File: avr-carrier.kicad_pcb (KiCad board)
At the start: 2 copper layers, 1 part

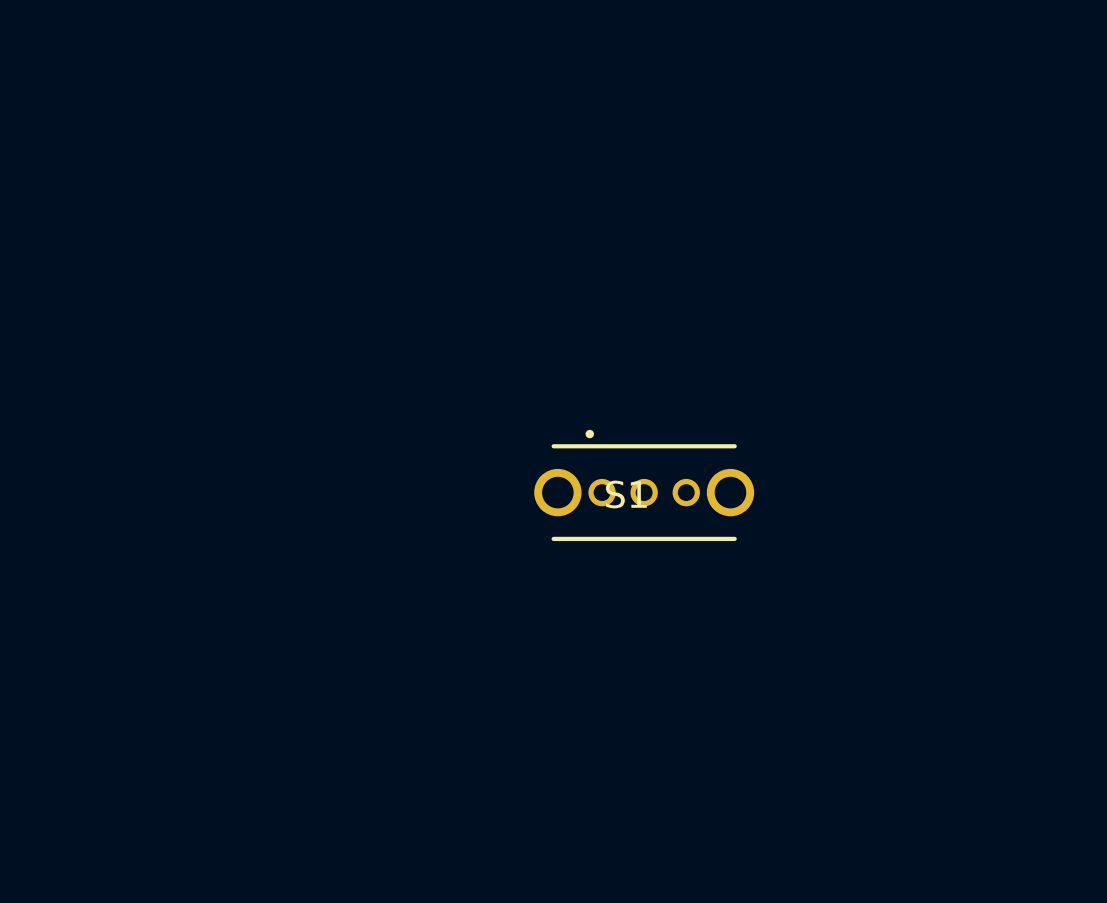
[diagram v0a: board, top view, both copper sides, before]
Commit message: hmm
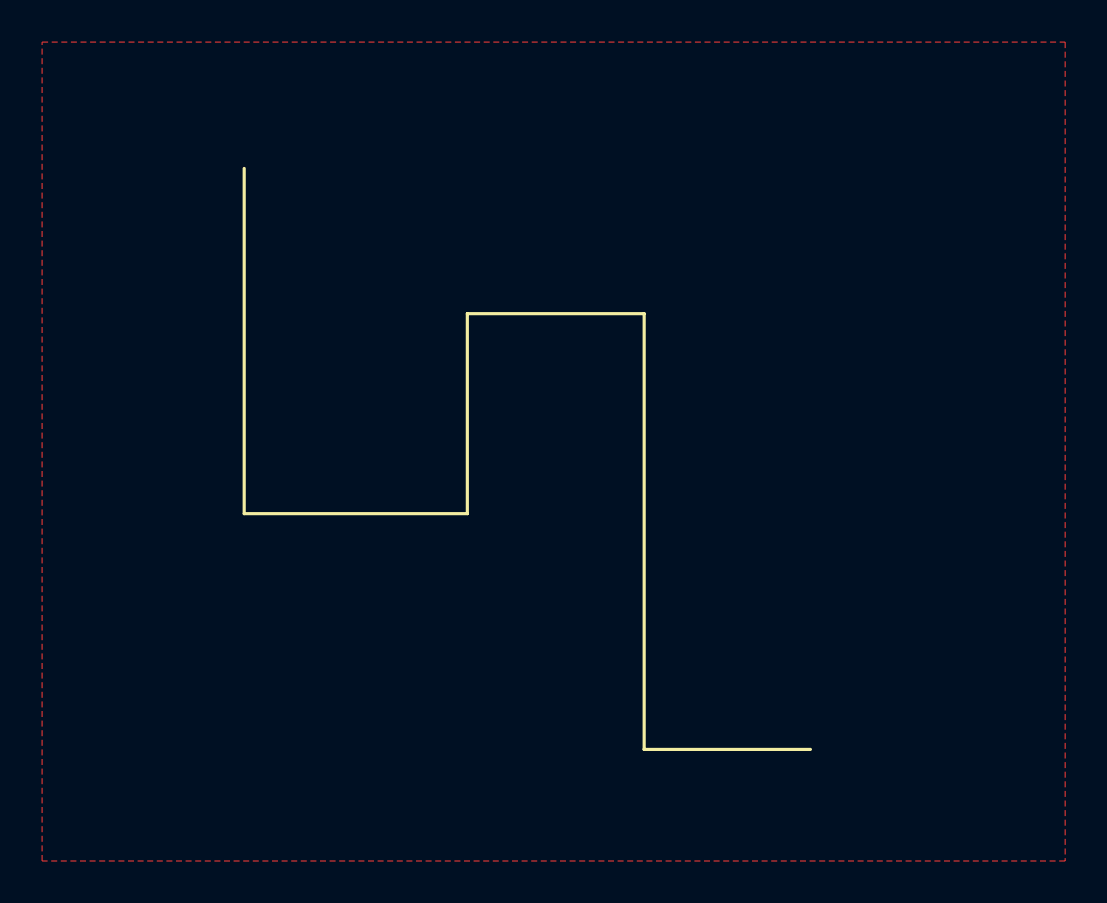
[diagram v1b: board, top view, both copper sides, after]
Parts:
- removed S1: OS102011MA1QN1, Switches_CC:OS102011MA1QN1
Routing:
- added copper zone on F.Cu, net (none)
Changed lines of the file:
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@@
   )
   (net 0 "")
-  (net 1 "unconnected-(S1-Pad1)")
-  (net 2 "unconnected-(S1-Pad2)")
-  (net 3 "unconnected-(S1-Pad3)")
-  (footprint "Switches_CC:OS102011MA1QN1" (layer "F.Cu")
-    (at 128.7 103.8)
-    (descr "OS102011MA1QN1")
-    (tags "Switch")
-    (property "Description" "Switch Slide Right Angle SPDT 0.1A 12VDC Through Hole Slide Switch SPDT On-On 0.1 A@ 12 V dc Slide")
-    (property "Height" "")
-    (property "Manufacturer_Name" "C & K COMPONENTS")
-    (property "Manufacturer_Part_Number" "OS102011MA1QN1")
-    (property "Mouser Part Number" "611-OS102011MA1QN1")
-    (property "Mouser Price/Stock" "https://www.mouser.co.uk/ProductDetail/CK/OS102011MA1QN1?qs=WtljUlYws5R6MUgHcLkz4w%3D%3D")
-    (property "Sheetfile" "avr-carrier.kicad_sch")
-    (property "Sheetname" "")
-    (attr through_hole)
-    (fp_text reference "S1" (at -0.822 0.137) (layer "F.SilkS")
-      (effects (font (size 1.27 1.27) (thickness 0.254)))
-    )
-    (fp_text value "OS102011MA1QN1" (at -0.822 0.137) (layer "F.SilkS") hide
-      (effects (font (size 1.27 1.27) (thickness 0.254)))
-    )
-    (fp_text user "${REFERENCE}" (at -0.822 0.137) (layer "F.Fab")
-      (effects (font (size 1.27 1.27) (thickness 0.254)))
-    )
-    (fp_line (start -4.3 -2.2) (end 4.3 -2.2) (layer "F.SilkS") (width 0.2))
-    (fp_line (start -4.3 2.2) (end 4.3 2.2) (layer "F.SilkS") (width 0.2))
-    (fp_circle (center -2.583 -2.781) (end -2.583 -2.68172) (layer "F.SilkS") (width 0.2) (fill none))
-    (fp_line (start -4.3 2.2) (end -4.3 -2.2) (layer "F.Fab") (width 0.2))
-    (fp_line (start -4.3 -2.2) (end 4.3 -2.2) (layer "F.Fab") (width 0.2))
-    (fp_line (start 4.3 -2.2) (end 4.3 2.2) (layer "F.Fab") (width 0.2))
-    (fp_line (start 4.3 2.2) (end -4.3 2.2) (layer "F.Fab") (width 0.2))
-    (pad "1" thru_hole circle (at -2 0) (size 1.3 1.3) (drill 0.8) (layers *.Cu *.Mask)
-      (net 1 "unconnected-(S1-Pad1)") (pinfunction "1") (pintype "passive"))
-    (pad "2" thru_hole circle (at 0 0) (size 1.3 1.3) (drill 0.8) (layers *.Cu *.Mask)
-      (net 2 "unconnected-(S1-Pad2)") (pinfunction "2") (pintype "passive"))
-    (pad "3" thru_hole circle (at 2 0) (size 1.3 1.3) (drill 0.8) (layers *.Cu *.Mask)
-      (net 3 "unconnected-(S1-Pad3)") (pinfunction "3") (pintype "passive"))
-    (pad "4" thru_hole circle (at -4.1 0) (size 2.25 2.25) (drill 1.5) (layers *.Cu *.Mask))
-    (pad "5" thru_hole circle (at 4.1 0) (size 2.25 2.25) (drill 1.5) (layers *.Cu *.Mask))
-    (model "${PCB_LIB_DIR}/3D/Switches_CC.3dshapes/OS102011MA1QN1.stp"
-      (offset (xyz -19.5 9.65 -20))
-      (scale (xyz 1 1 1))
-      (rotate (xyz -90 0 -180))
+  (gr_line (start 128.7 95.3) (end 128.7 116) (layer "F.SilkS") (width 0.15))
+  (gr_line (start 128.7 116) (end 136.6 116) (layer "F.SilkS") (width 0.15))
+  (gr_line (start 109.7 88.4) (end 109.7 104.8) (layer "F.SilkS") (width 0.15))
+  (gr_line (start 120.3 95.3) (end 128.7 95.3) (layer "F.SilkS") (width 0.15))
+  (gr_line (start 120.3 104.8) (end 120.3 95.3) (layer "F.SilkS") (width 0.15))
+  (gr_line (start 109.7 104.8) (end 120.3 104.8) (layer "F.SilkS") (width 0.15))
+  (zone (net 0) (net_name "") (layer "F.Cu") (hatch edge 0.508)
+    (connect_pads (clearance 0.508))
+    (min_thickness 0.254) (filled_areas_thickness no)
+    (fill yes (thermal_gap 0.508) (thermal_bridge_width 0.508))
+    (polygon
+      (pts
+        (xy 148.7 121.3)
+        (xy 100.1 121.3)
+        (xy 100.1 82.4)
+        (xy 148.7 82.4)
+      )
     )
   )
